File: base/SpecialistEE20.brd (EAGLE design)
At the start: 55.9 x 6.6 mm, 105 parts, among them X1 SCART-F

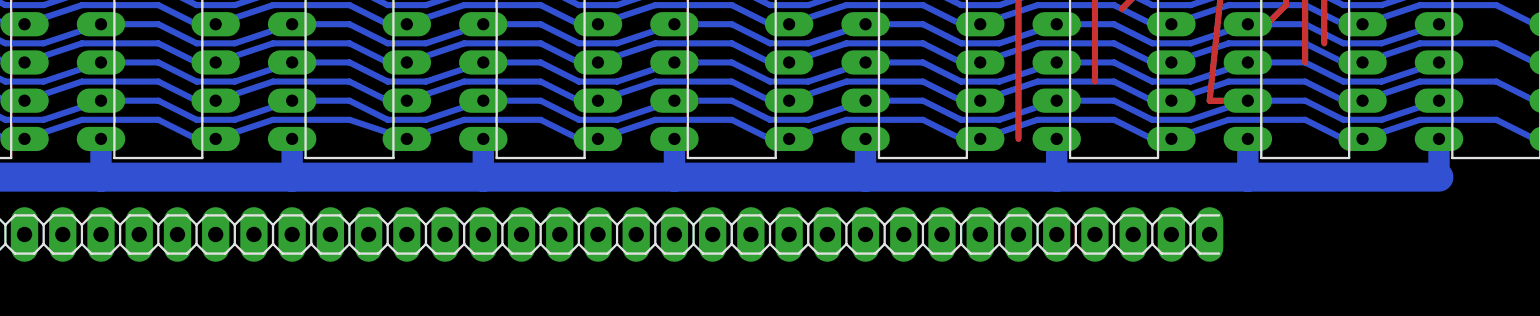
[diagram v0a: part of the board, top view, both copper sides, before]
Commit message: .
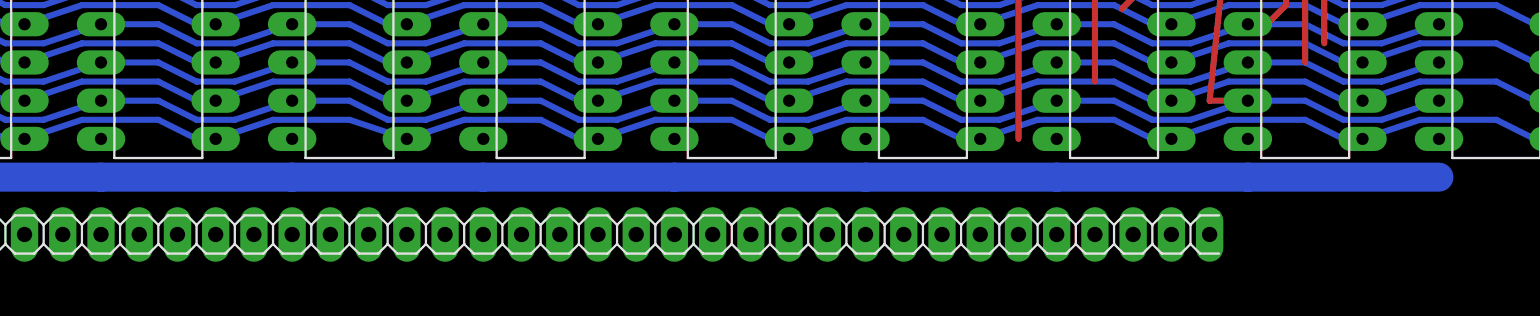
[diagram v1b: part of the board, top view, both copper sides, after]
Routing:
- net +5V: track 211.1 -> 190.8 mm
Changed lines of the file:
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@@
 <contactref element="RD1" pad="2"/>
 <contactref element="RD2" pad="1"/>
-<contactref element="DD21" pad="8"/>
-<contactref element="DD28" pad="8"/>
-<contactref element="DD27" pad="8"/>
-<contactref element="DD26" pad="8"/>
-<contactref element="DD25" pad="8"/>
-<contactref element="DD24" pad="8"/>
-<contactref element="DD23" pad="8"/>
-<contactref element="DD22" pad="8"/>
 <contactref element="DD102" pad="8"/>
 <contactref element="DD103" pad="8"/>
@@
 <wire x1="49.53" y1="1.27" x2="38.1" y2="1.27" width="1.9304" layer="16"/>
 <wire x1="38.1" y1="1.27" x2="25.4" y2="1.27" width="1.9304" layer="16"/>
-<wire x1="63.5" y1="3.81" x2="63.5" y2="1.27" width="1.4224" layer="16"/>
-<wire x1="76.2" y1="3.81" x2="76.2" y2="1.27" width="1.4224" layer="16"/>
-<wire x1="88.9" y1="3.81" x2="88.9" y2="1.27" width="1.4224" layer="16"/>
-<wire x1="101.6" y1="3.81" x2="101.6" y2="1.27" width="1.4224" layer="16"/>
-<wire x1="114.3" y1="3.81" x2="114.3" y2="1.27" width="1.4224" layer="16"/>
-<wire x1="127" y1="3.81" x2="127" y2="1.27" width="1.4224" layer="16"/>
-<wire x1="139.7" y1="3.81" x2="139.7" y2="1.27" width="1.4224" layer="16"/>
-<wire x1="152.4" y1="1.27" x2="152.4" y2="3.81" width="1.4224" layer="16"/>
 <contactref element="R106" pad="2"/>
 <contactref element="R105" pad="2"/>
@@
 <contactref element="DD107" pad="14"/>
 <contactref element="DD112" pad="26"/>
+<contactref element="DD21" pad="8"/>
+<contactref element="DD22" pad="8"/>
+<contactref element="DD23" pad="8"/>
+<contactref element="DD24" pad="8"/>
+<contactref element="DD28" pad="8"/>
+<contactref element="DD27" pad="8"/>
+<contactref element="DD26" pad="8"/>
+<contactref element="DD25" pad="8"/>
 <wire x1="125.6" y1="107.95" x2="124.33" y2="115.57" width="0" layer="19" extent="1-16"/>
 <wire x1="116.84" y1="107.95" x2="125.6" y2="107.95" width="0" layer="19" extent="16-16"/>
@@
 <wire x1="208.6" y1="-6.35" x2="207.33" y2="-5.08" width="0" layer="19" extent="16-16"/>
 <wire x1="152.4" y1="1.27" x2="207.33" y2="-5.08" width="0" layer="19" extent="16-16"/>
+<wire x1="152.4" y1="3.81" x2="152.4" y2="1.27" width="0" layer="19" extent="16-16"/>
+<wire x1="139.7" y1="3.81" x2="139.7" y2="1.27" width="0" layer="19" extent="16-16"/>
+<wire x1="127" y1="3.81" x2="127" y2="1.27" width="0" layer="19" extent="16-16"/>
+<wire x1="114.3" y1="3.81" x2="114.3" y2="1.27" width="0" layer="19" extent="16-16"/>
+<wire x1="101.6" y1="3.81" x2="101.6" y2="1.27" width="0" layer="19" extent="16-16"/>
+<wire x1="88.9" y1="3.81" x2="88.9" y2="1.27" width="0" layer="19" extent="16-16"/>
+<wire x1="76.2" y1="3.81" x2="76.2" y2="1.27" width="0" layer="19" extent="16-16"/>
+<wire x1="63.5" y1="3.81" x2="63.5" y2="1.27" width="0" layer="19" extent="16-16"/>
 <wire x1="274.32" y1="-15.37" x2="208.6" y2="-6.35" width="0" layer="19" extent="16-16"/>
 <wire x1="307.34" y1="17.78" x2="274.32" y2="-15.37" width="0" layer="19" extent="16-16"/>
